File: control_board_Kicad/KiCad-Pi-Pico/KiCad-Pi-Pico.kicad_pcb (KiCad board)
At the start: 2 copper layers, 100 x 70 mm, 25 parts, among them J1 DB25_Plug_MountingHoles, Q1 2N7002, Q2 2N7002, Q3 2N7002, Q4 2N7002, SW1 SW_Push, U1 SC0915, U2 AD5761RBRUZ, U3 LM285D-2.5

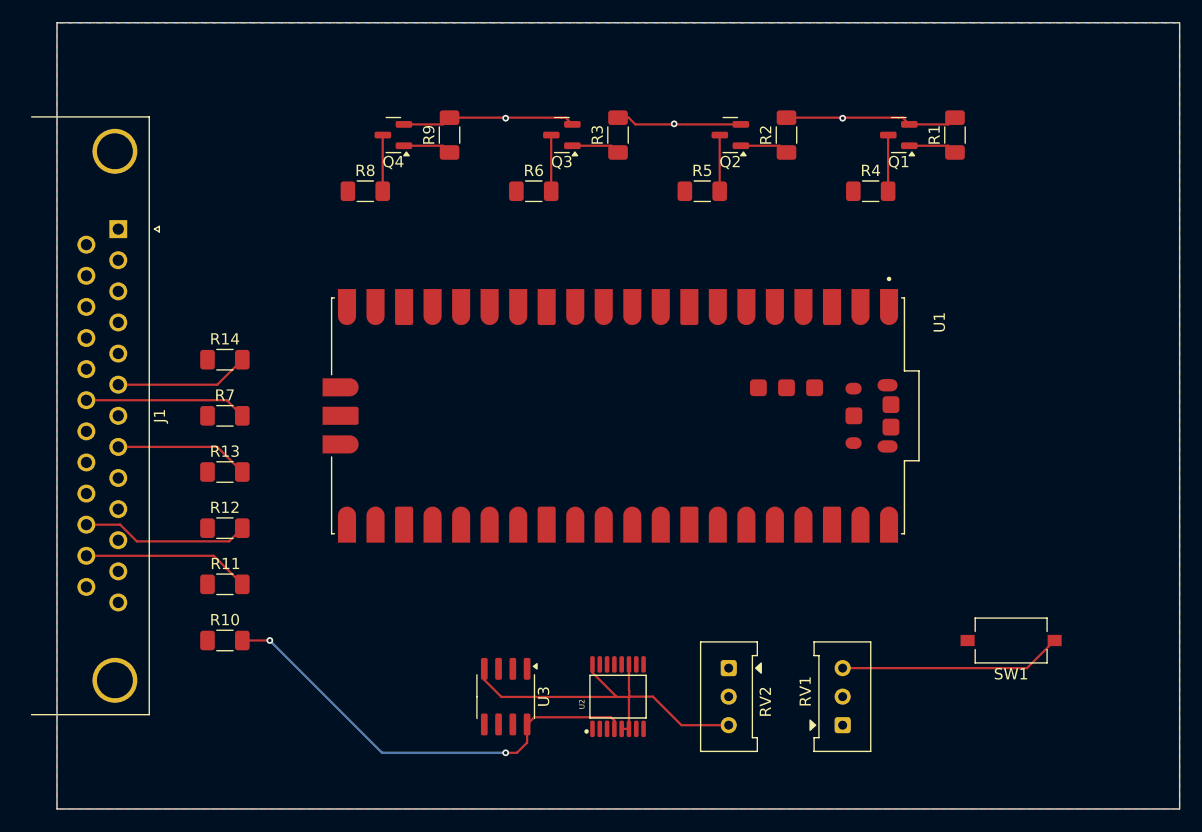
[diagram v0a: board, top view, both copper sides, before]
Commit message: KiCad updated
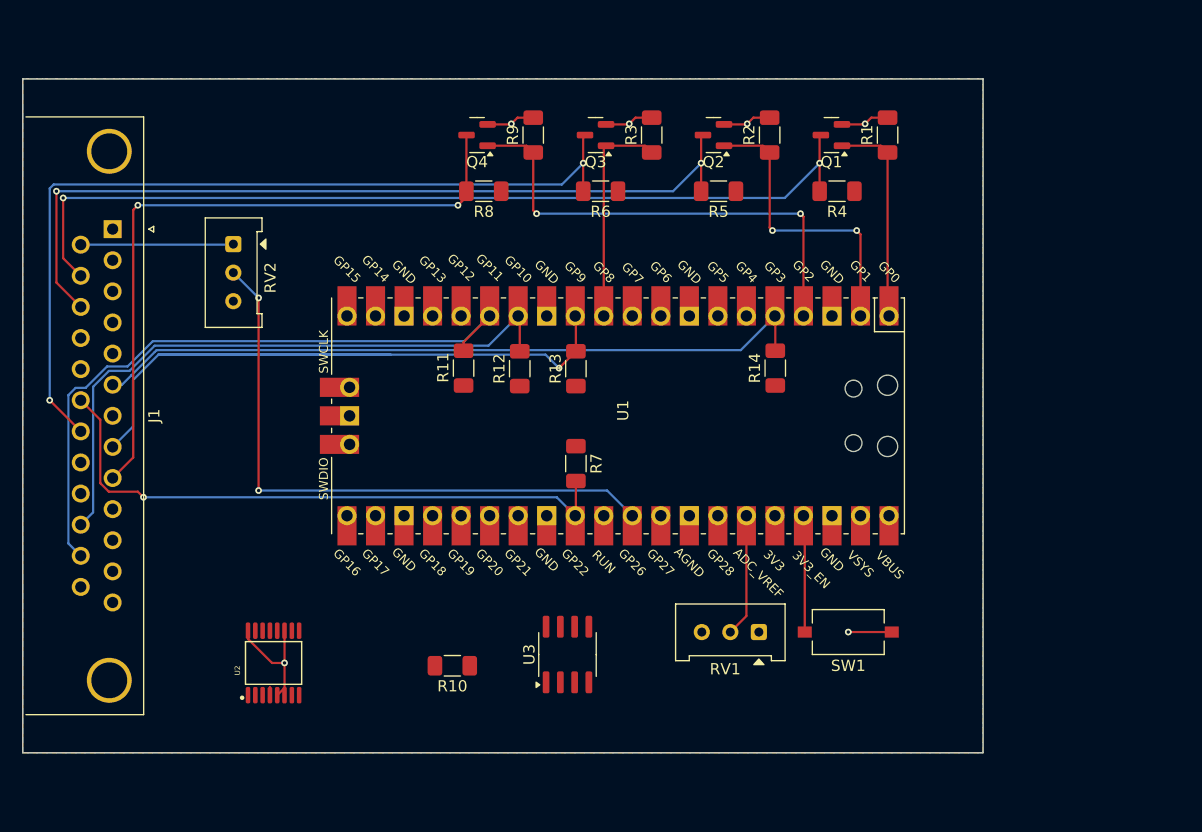
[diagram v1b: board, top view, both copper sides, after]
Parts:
- U1: footprint SC0915:MODULE_SC0915 -> RPi_Pico:RPi_Pico_SMD_TH
- moved RV2 58.1 mm to (115.8, 84.7)
- moved R14 49.0 mm to (164.0, 95.8), turned to 90 degrees
- moved R13 32.6 mm to (146.2, 95.8), turned to 90 degrees
- moved R7 31.5 mm to (146.2, 104.2), turned to -90 degrees
- moved U2 30.8 mm to (119.3, 122.0)
- moved R12 29.8 mm to (141.2, 95.8), turned to 90 degrees
- moved R11 28.7 mm to (136.2, 95.8), turned to 90 degrees
- moved R10 20.4 mm to (135.2, 122.2), turned to 180 degrees
- moved SW1 14.5 mm to (170.5, 119.2)
- moved RV1 11.2 mm to (162.5, 119.2), turned to 180 degrees
- moved R8 10.6 mm to (138.1, 80.0), turned to 180 degrees
- moved Q4 7.45 mm to (137.4, 75.0)
- moved R9 7.45 mm to (142.4, 75.0)
- moved U3 6.66 mm to (145.5, 121.2), turned to 90 degrees
- moved Q1 6.00 mm to (169.0, 75.0)
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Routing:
- net Net-(U1-GP9): track 12.0 -> 92.7 mm, vias 0 -> 1
- net Net-(J1-P15): track 5.01 -> 81.3 mm, vias 0 -> 2
- net Net-(J1-P20): track 5.01 -> 76.3 mm, vias 0 -> 2
- net Net-(J1-P16): track 5.01 -> 74.7 mm, vias 0 -> 2
- net GND: track 97.3 -> 32.5 mm, vias 3 -> 6
- net Net-(Q4-D): track 5.01 -> 60.3 mm, vias 0 -> 2
- net Net-(U1-GP26): track 0.00 -> 54.5 mm, vias 0 -> 2
- net Net-(U1-GP3): track 12.0 -> 64.6 mm
- net Net-(J1-P24): track 14.9 -> 59.2 mm
- net Net-(J1-P23): track 15.0 -> 56.4 mm
- net Net-(J1-P19): track 14.5 -> 55.5 mm, vias 0 -> 1
- net +2V5REF: track 40.4 -> 0.73 mm, vias 2 -> 0
- net Net-(Q4-G): track 4.31 -> 42.6 mm, vias 0 -> 2
- net Net-(Q2-G): track 4.31 -> 26.6 mm, vias 0 -> 2
- net Net-(Q3-G): track 4.31 -> 19.6 mm
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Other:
- board size 100 x 70 mm -> 85.5 x 60 mm
